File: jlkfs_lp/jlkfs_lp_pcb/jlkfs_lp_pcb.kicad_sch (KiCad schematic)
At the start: 40 parts, among them J0 USB_C_Receptacle_PowerOnly_6P, SW0 SWITCH, SW1 SWITCH, SW10 SWITCH, SW11 SWITCH, SW12 SWITCH, SW13 SWITCH, SW14 SWITCH, SW15 SWITCH, SW16 SWITCH, SW17 SWITCH, SW18 SWITCH, SW19 SWITCH, SW2 SWITCH, SW20 SWITCH, SW21 SWITCH, SW22 SWITCH, SW23 SWITCH, SW24 SWITCH, SW25 SWITCH, SW26 SWITCH, SW27 SWITCH, SW28 SWITCH, SW3 SWITCH, SW4 SWITCH, SW5 SWITCH, SW6 SWITCH, SW7 SWITCH, SW8 SWITCH, SW9 SWITCH, U0 RP2040

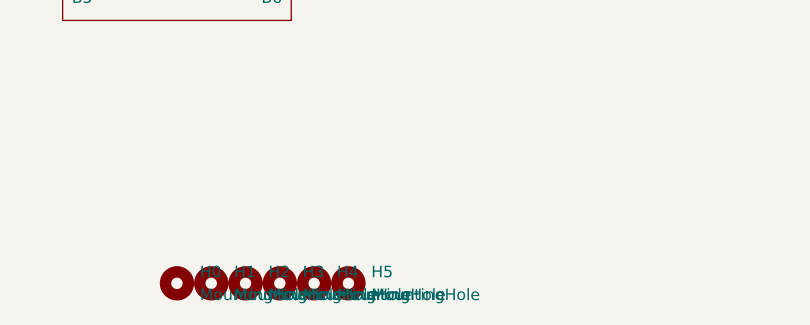
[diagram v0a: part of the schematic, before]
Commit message: Updates to jlkfs_lp.
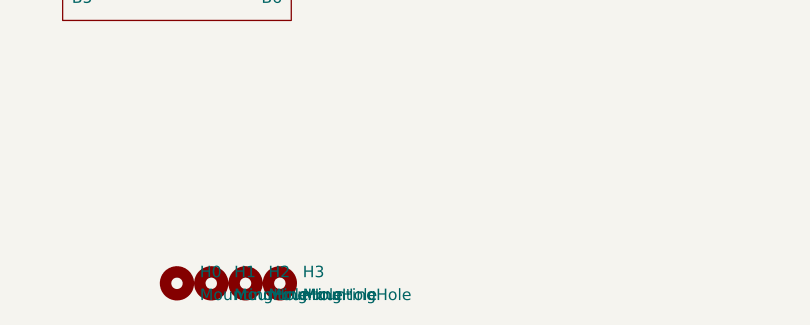
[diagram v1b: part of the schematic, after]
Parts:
- removed H4, H5: MountingHole, MountingHole:MountingHole_3.5mm, symbol Mechanical:MountingHole
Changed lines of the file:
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@@
     (pin "11")
     (instances
-      (project "jlkfs_lower"
+      (project "jlkfs_lp_pcb"
         (path "/97127b28-60f4-45ff-835e-dccfbc833331"
           (reference "U0") (unit 1)
@@
     (pin "2")
     (instances
-      (project "jlkfs_lower"
+      (project "jlkfs_lp_pcb"
         (path "/97127b28-60f4-45ff-835e-dccfbc833331"
           (reference "SW13") (unit 1)
@@
     )
   )
-  (symbol (lib_id "Mechanical:MountingHole") (at 134.62 250.19 0) (unit 1)
-    (in_bom yes) (on_board yes) (dnp no) (fields_autoplaced)
-    (property "Reference" "H4" (at 137.16 248.92 0)
-      (effects (font (size 1.27 1.27)) (justify left))
-    )
-    (property "Value" "MountingHole" (at 137.16 251.46 0)
-      (effects (font (size 1.27 1.27)) (justify left))
-    )
-    (property "Footprint" "MountingHole:MountingHole_3.5mm" (at 134.62 250.19 0)
-      (effects (font (size 1.27 1.27)) hide)
-    )
-    (property "Datasheet" "~" (at 134.62 250.19 0)
-      (effects (font (size 1.27 1.27)) hide)
-    )
-    (instances
-      (project "jlkfs_lower"
-        (path "/97127b28-60f4-45ff-835e-dccfbc833331"
-          (reference "H4") (unit 1)
-        )
-      )
-    )
-  )
   (symbol (lib_id "symbols:SWITCH_WITH_DIODE") (at 198.12 77.47 0) (unit 1)
     (in_bom yes) (on_board yes) (dnp no) (fields_autoplaced)
@@
     (pin "2")
     (instances
-      (project "jlkfs_lower"
+      (project "jlkfs_lp_pcb"
         (path "/97127b28-60f4-45ff-835e-dccfbc833331"
           (reference "SW11") (unit 1)
@@
     (pin "2")
     (instances
-      (project "jlkfs_lower"
+      (project "jlkfs_lp_pcb"
         (path "/97127b28-60f4-45ff-835e-dccfbc833331"
           (reference "SW23") (unit 1)
@@
     (pin "2")
     (instances
-      (project "jlkfs_lower"
+      (project "jlkfs_lp_pcb"
         (path "/97127b28-60f4-45ff-835e-dccfbc833331"
           (reference "SW14") (unit 1)
@@
     (pin "2")
     (instances
-      (project "jlkfs_lower"
+      (project "jlkfs_lp_pcb"
         (path "/97127b28-60f4-45ff-835e-dccfbc833331"
           (reference "SW20") (unit 1)
@@
     (pin "2")
     (instances
-      (project "jlkfs_lower"
+      (project "jlkfs_lp_pcb"
         (path "/97127b28-60f4-45ff-835e-dccfbc833331"
           (reference "SW10") (unit 1)
@@
     (pin "2")
     (instances
-      (project "jlkfs_lower"
+      (project "jlkfs_lp_pcb"
         (path "/97127b28-60f4-45ff-835e-dccfbc833331"
           (reference "SW27") (unit 1)
@@
     (pin "2")
     (instances
-      (project "jlkfs_lower"
+      (project "jlkfs_lp_pcb"
         (path "/97127b28-60f4-45ff-835e-dccfbc833331"
           (reference "SW15") (unit 1)
@@
     (pin "2")
     (instances
-      (project "jlkfs_lower"
+      (project "jlkfs_lp_pcb"
         (path "/97127b28-60f4-45ff-835e-dccfbc833331"
           (reference "SW1") (unit 1)
@@
     (pin "2")
     (instances
-      (project "jlkfs_lower"
+      (project "jlkfs_lp_pcb"
         (path "/97127b28-60f4-45ff-835e-dccfbc833331"
           (reference "SW18") (unit 1)
@@
     (pin "2")
     (instances
-      (project "jlkfs_lower"
+      (project "jlkfs_lp_pcb"
         (path "/97127b28-60f4-45ff-835e-dccfbc833331"
           (reference "SW8") (unit 1)
@@
     (pin "2")
     (instances
-      (project "jlkfs_lower"
+      (project "jlkfs_lp_pcb"
         (path "/97127b28-60f4-45ff-835e-dccfbc833331"
           (reference "SW4") (unit 1)
@@
     (pin "2")
     (instances
-      (project "jlkfs_lower"
+      (project "jlkfs_lp_pcb"
         (path "/97127b28-60f4-45ff-835e-dccfbc833331"
           (reference "SW16") (unit 1)
@@
     (pin "2")
     (instances
-      (project "jlkfs_lower"
+      (project "jlkfs_lp_pcb"
         (path "/97127b28-60f4-45ff-835e-dccfbc833331"
           (reference "SW22") (unit 1)
@@
     (pin "2")
     (instances
-      (project "jlkfs_lower"
+      (project "jlkfs_lp_pcb"
         (path "/97127b28-60f4-45ff-835e-dccfbc833331"
           (reference "SW2") (unit 1)
@@
     (pin "2")
     (instances
-      (project "jlkfs_lower"
+      (project "jlkfs_lp_pcb"
         (path "/97127b28-60f4-45ff-835e-dccfbc833331"
           (reference "SW0") (unit 1)
@@
     )
     (instances
-      (project "jlkfs_lower"
+      (project "jlkfs_lp_pcb"
         (path "/97127b28-60f4-45ff-835e-dccfbc833331"
           (reference "H0") (unit 1)
@@
     (pin "2")
     (instances
-      (project "jlkfs_lower"
+      (project "jlkfs_lp_pcb"
         (path "/97127b28-60f4-45ff-835e-dccfbc833331"
           (reference "SW12") (unit 1)
@@
     )
     (instances
-      (project "jlkfs_lower"
+      (project "jlkfs_lp_pcb"
         (path "/97127b28-60f4-45ff-835e-dccfbc833331"
           (reference "H3") (unit 1)
@@
     (pin "1")
     (instances
-      (project "jlkfs_lower"
+      (project "jlkfs_lp_pcb"
         (path "/97127b28-60f4-45ff-835e-dccfbc833331"
           (reference "#PWR01") (unit 1)
@@
     (pin "2")
     (instances
-      (project "jlkfs_lower"
+      (project "jlkfs_lp_pcb"
         (path "/97127b28-60f4-45ff-835e-dccfbc833331"
           (reference "SW5") (unit 1)
@@
     (pin "2")
     (instances
-      (project "jlkfs_lower"
+      (project "jlkfs_lp_pcb"
         (path "/97127b28-60f4-45ff-835e-dccfbc833331"
           (reference "R1") (unit 1)
@@
     (pin "1")
     (instances
-      (project "jlkfs_lower"
+      (project "jlkfs_lp_pcb"
         (path "/97127b28-60f4-45ff-835e-dccfbc833331"
           (reference "#PWR02") (unit 1)
@@
     (pin "2")
     (instances
-      (project "jlkfs_lower"
+      (project "jlkfs_lp_pcb"
         (path "/97127b28-60f4-45ff-835e-dccfbc833331"
           (reference "SW7") (unit 1)
@@
     (pin "2")
     (instances
-      (project "jlkfs_lower"
+      (project "jlkfs_lp_pcb"
         (path "/97127b28-60f4-45ff-835e-dccfbc833331"
           (reference "SW9") (unit 1)
@@
     (pin "2")
     (instances
-      (project "jlkfs_lower"
+      (project "jlkfs_lp_pcb"
         (path "/97127b28-60f4-45ff-835e-dccfbc833331"
           (reference "SW3") (unit 1)
@@
     (pin "2")
     (instances
-      (project "jlkfs_lower"
+      (project "jlkfs_lp_pcb"
         (path "/97127b28-60f4-45ff-835e-dccfbc833331"
           (reference "SW26") (unit 1)
@@
     )
     (instances
-      (project "jlkfs_lower"
+      (project "jlkfs_lp_pcb"
         (path "/97127b28-60f4-45ff-835e-dccfbc833331"
           (reference "H2") (unit 1)
@@
     (pin "1")
     (instances
-      (project "jlkfs_lower"
+      (project "jlkfs_lp_pcb"
         (path "/97127b28-60f4-45ff-835e-dccfbc833331"
           (reference "#PWR00") (unit 1)
@@
     (pin "2")
     (instances
-      (project "jlkfs_lower"
+      (project "jlkfs_lp_pcb"
         (path "/97127b28-60f4-45ff-835e-dccfbc833331"
           (reference "SW24") (unit 1)
@@
     (pin "2")
     (instances
-      (project "jlkfs_lower"
+      (project "jlkfs_lp_pcb"
         (path "/97127b28-60f4-45ff-835e-dccfbc833331"
           (reference "SW28") (unit 1)
@@
     (pin "2")
     (instances
-      (project "jlkfs_lower"
+      (project "jlkfs_lp_pcb"
         (path "/97127b28-60f4-45ff-835e-dccfbc833331"
           (reference "R0") (unit 1)
@@
     (pin "2")
     (instances
-      (project "jlkfs_lower"
+      (project "jlkfs_lp_pcb"
         (path "/97127b28-60f4-45ff-835e-dccfbc833331"
           (reference "SW21") (unit 1)
@@
     )
     (instances
-      (project "jlkfs_lower"
+      (project "jlkfs_lp_pcb"
         (path "/97127b28-60f4-45ff-835e-dccfbc833331"
           (reference "H1") (unit 1)
@@
     (pin "2")
     (instances
-      (project "jlkfs_lower"
+      (project "jlkfs_lp_pcb"
         (path "/97127b28-60f4-45ff-835e-dccfbc833331"
           (reference "SW6") (unit 1)
@@
     (pin "2")
     (instances
-      (project "jlkfs_lower"
+      (project "jlkfs_lp_pcb"
         (path "/97127b28-60f4-45ff-835e-dccfbc833331"
           (reference "SW25") (unit 1)
@@
     (pin "A12")
     (instances
-      (project "jlkfs_lower"
+      (project "jlkfs_lp_pcb"
         (path "/97127b28-60f4-45ff-835e-dccfbc833331"
           (reference "J0") (unit 1)
@@
     (pin "2")
     (instances
-      (project "jlkfs_lower"
+      (project "jlkfs_lp_pcb"
         (path "/97127b28-60f4-45ff-835e-dccfbc833331"
           (reference "SW17") (unit 1)
@@
     (pin "2")
     (instances
-      (project "jlkfs_lower"
+      (project "jlkfs_lp_pcb"
         (path "/97127b28-60f4-45ff-835e-dccfbc833331"
           (reference "RST0") (unit 1)
@@
     )
   )
-  (symbol (lib_id "Mechanical:MountingHole") (at 138.43 250.19 0) (unit 1)
-    (in_bom yes) (on_board yes) (dnp no) (fields_autoplaced)
-    (property "Reference" "H5" (at 140.97 248.92 0)
-      (effects (font (size 1.27 1.27)) (justify left))
-    )
-    (property "Value" "MountingHole" (at 140.97 251.46 0)
-      (effects (font (size 1.27 1.27)) (justify left))
-    )
-    (property "Footprint" "MountingHole:MountingHole_3.5mm" (at 138.43 250.19 0)
-      (effects (font (size 1.27 1.27)) hide)
-    )
-    (property "Datasheet" "~" (at 138.43 250.19 0)
-      (effects (font (size 1.27 1.27)) hide)
-    )
-    (instances
-      (project "jlkfs_lower"
-        (path "/97127b28-60f4-45ff-835e-dccfbc833331"
-          (reference "H5") (unit 1)
-        )
-      )
-    )
-  )
   (symbol (lib_id "symbols:SWITCH_WITH_DIODE") (at 30.48 105.41 0) (unit 1)
     (in_bom yes) (on_board yes) (dnp no) (fields_autoplaced)
@@
     (pin "2")
     (instances
-      (project "jlkfs_lower"
+      (project "jlkfs_lp_pcb"
         (path "/97127b28-60f4-45ff-835e-dccfbc833331"
           (reference "SW19") (unit 1)
